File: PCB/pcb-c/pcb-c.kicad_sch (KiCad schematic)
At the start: 37 parts, among them Q1 BC817, Q13 TPCA8120,L1Q, Q2 TPCA8120,L1Q, Q3 BC817, Q4 BC817, Q5 TPCA8120,L1Q, Q6 BC817, Q7 TPCA8120,L1Q, Q8 BC817, Q9 TPCA8120,L1Q

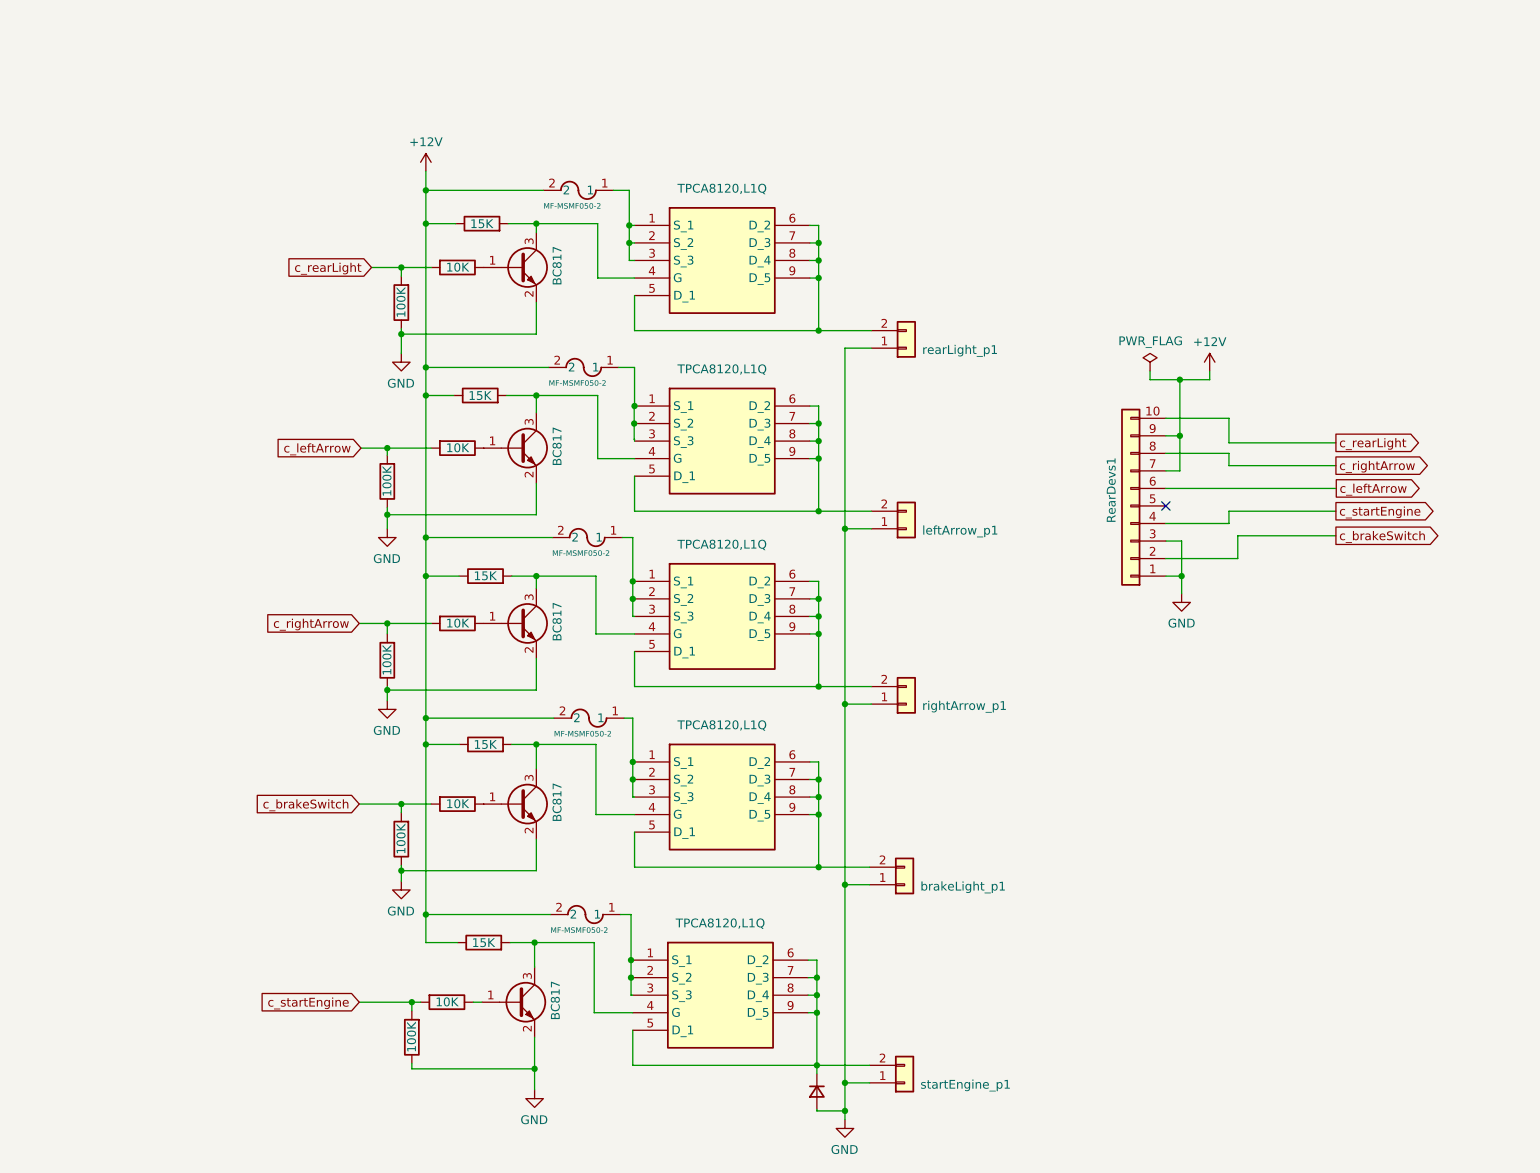
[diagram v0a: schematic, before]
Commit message: Mesge from ESP32__dualPCB
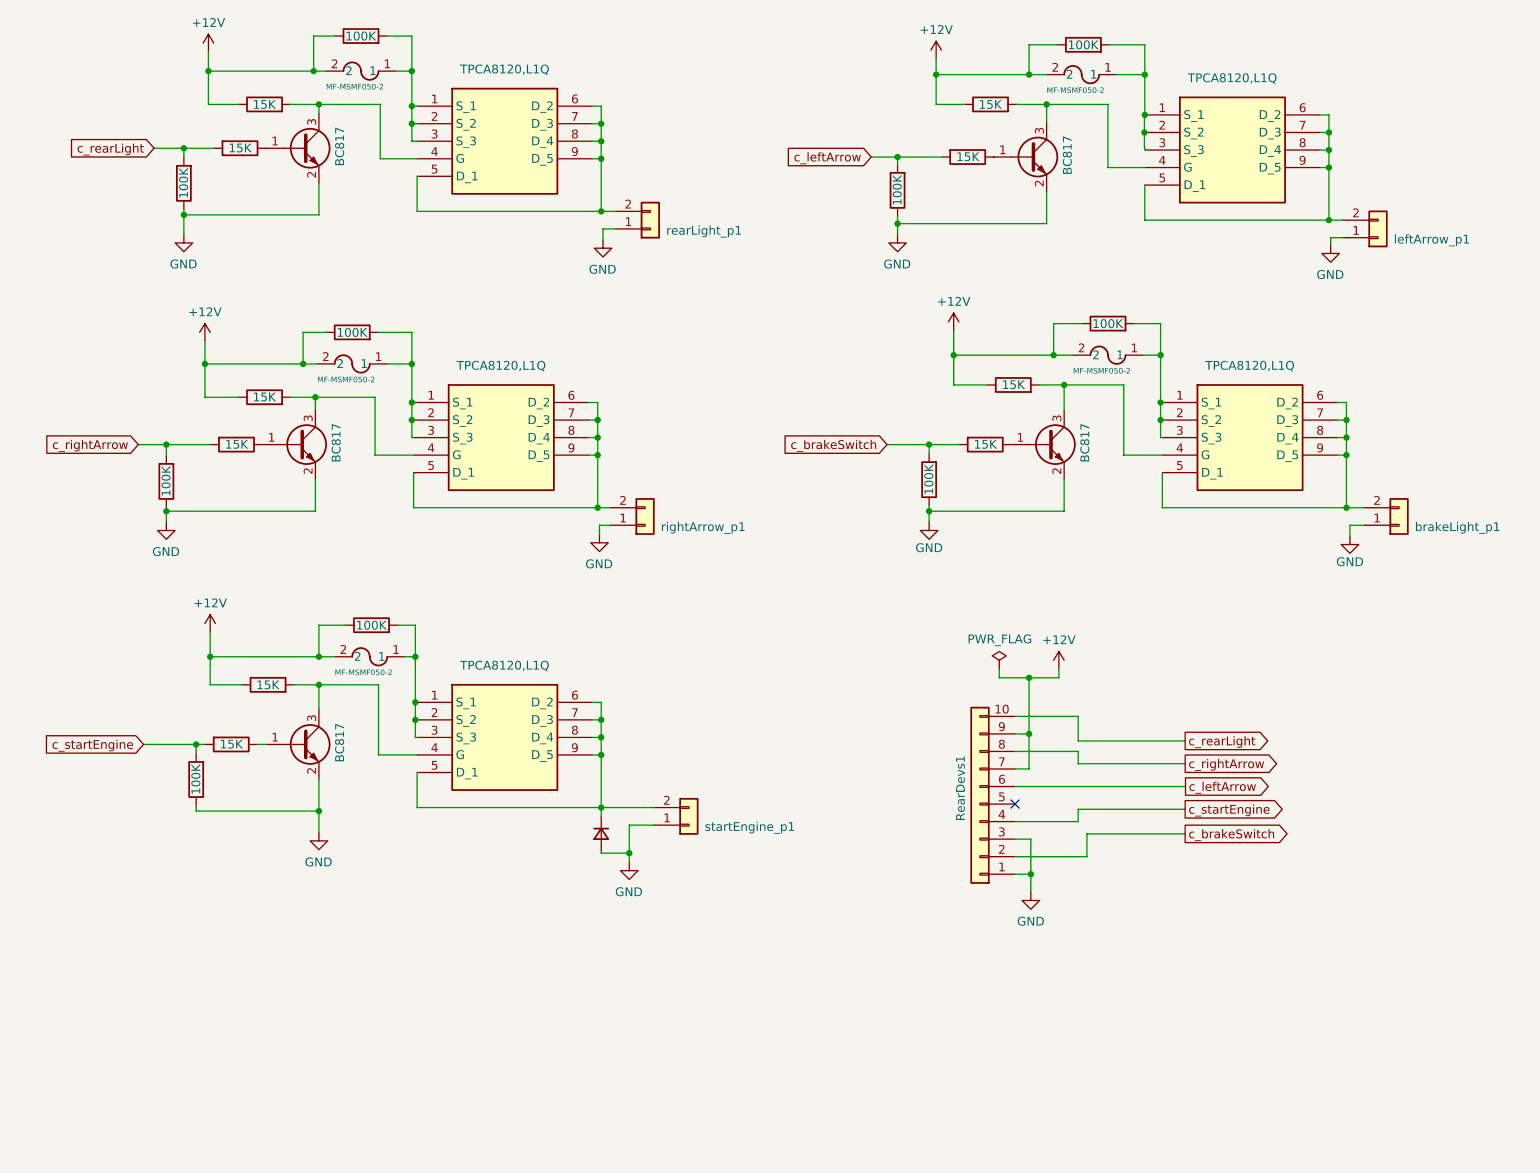
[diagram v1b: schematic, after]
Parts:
- added R11, R15, R19, R3, R6: 100K, Resistor_SMD:R_1206_3216Metric, symbol Device:R
- R13, R17, R4, R7, R9: value 10K -> 15K
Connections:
- net +12V: now also R11.1, R15.1, R19.1, R3.1, R6.1
- net at F3.1, Q13.1 (S_1), Q13.2 (S_2)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: now also R19.2
- net at F5.1, Q5.1 (S_1), Q5.2 (S_2)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: now also R3.2
- net at F4.1, Q7.1 (S_1), Q7.2 (S_2)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: now also R15.2
- net at F2.1, Q2.1 (S_1), Q2.2 (S_2)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: now also R6.2
- net at F1.1, Q9.1 (S_1), Q9.2 (S_2)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: now also R11.2
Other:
- moved on the sheet: RearDevs1, brakeLight_p1, leftArrow_p1, rearLight_p1, rightArrow_p1, startEngine_p1
